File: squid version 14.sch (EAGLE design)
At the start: 61 parts, among them J2 ATMEL_PROGRAMMER_HEADERNL, U2 MCP73832

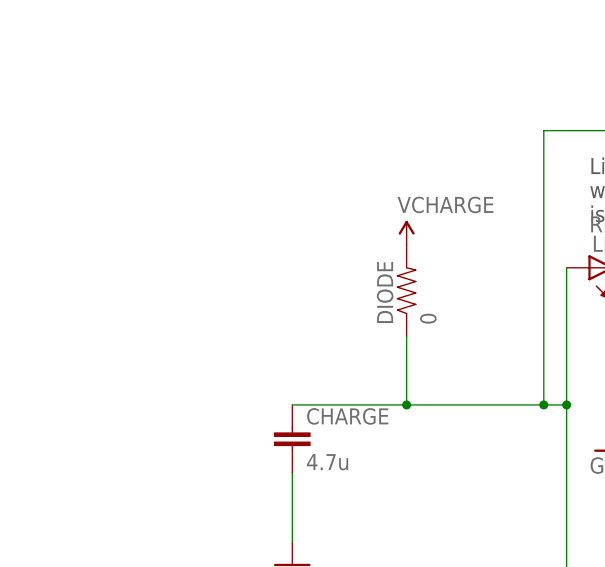
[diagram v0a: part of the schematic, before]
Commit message: add label
minor change
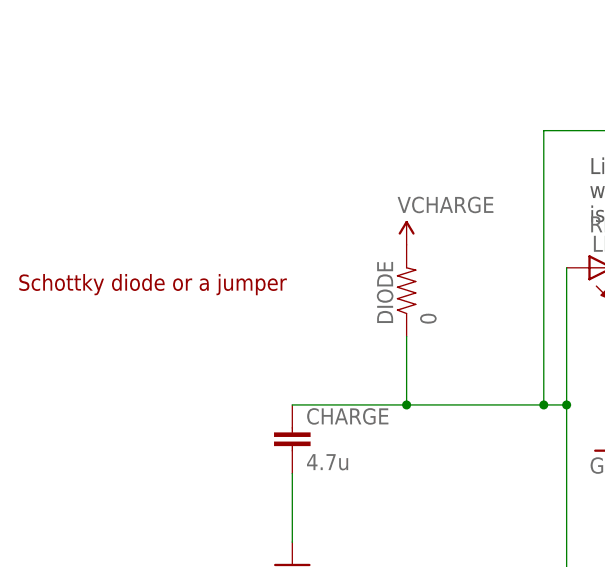
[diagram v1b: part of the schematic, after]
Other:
- note added: "Schottky diode or a jumper"
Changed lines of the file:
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@@
 <text x="109.22" y="190.5" size="1.778" layer="91">RESET LOW when charging</text>
 <text x="330.2" y="167.64" size="1.778" layer="94">Use a Resistor Array instead of discrete chips</text>
+<text x="-7.62" y="160.02" size="1.778" layer="94">Schottky diode or a jumper</text>
 </plain>
 <instances>
